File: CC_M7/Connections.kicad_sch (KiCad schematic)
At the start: 11 parts, among them J11 USB_B_Micro, J12 Conn_01x05_Pin, J16 Conn_01x06_Pin, J17 Conn_01x04_Pin, J3 Conn_01x03_Pin, J4 Conn_01x03_Pin, J5 Conn_01x03_Pin, J6 Conn_01x03_Pin, J7 Conn_01x03_Pin, J8 Conn_01x03_Pin

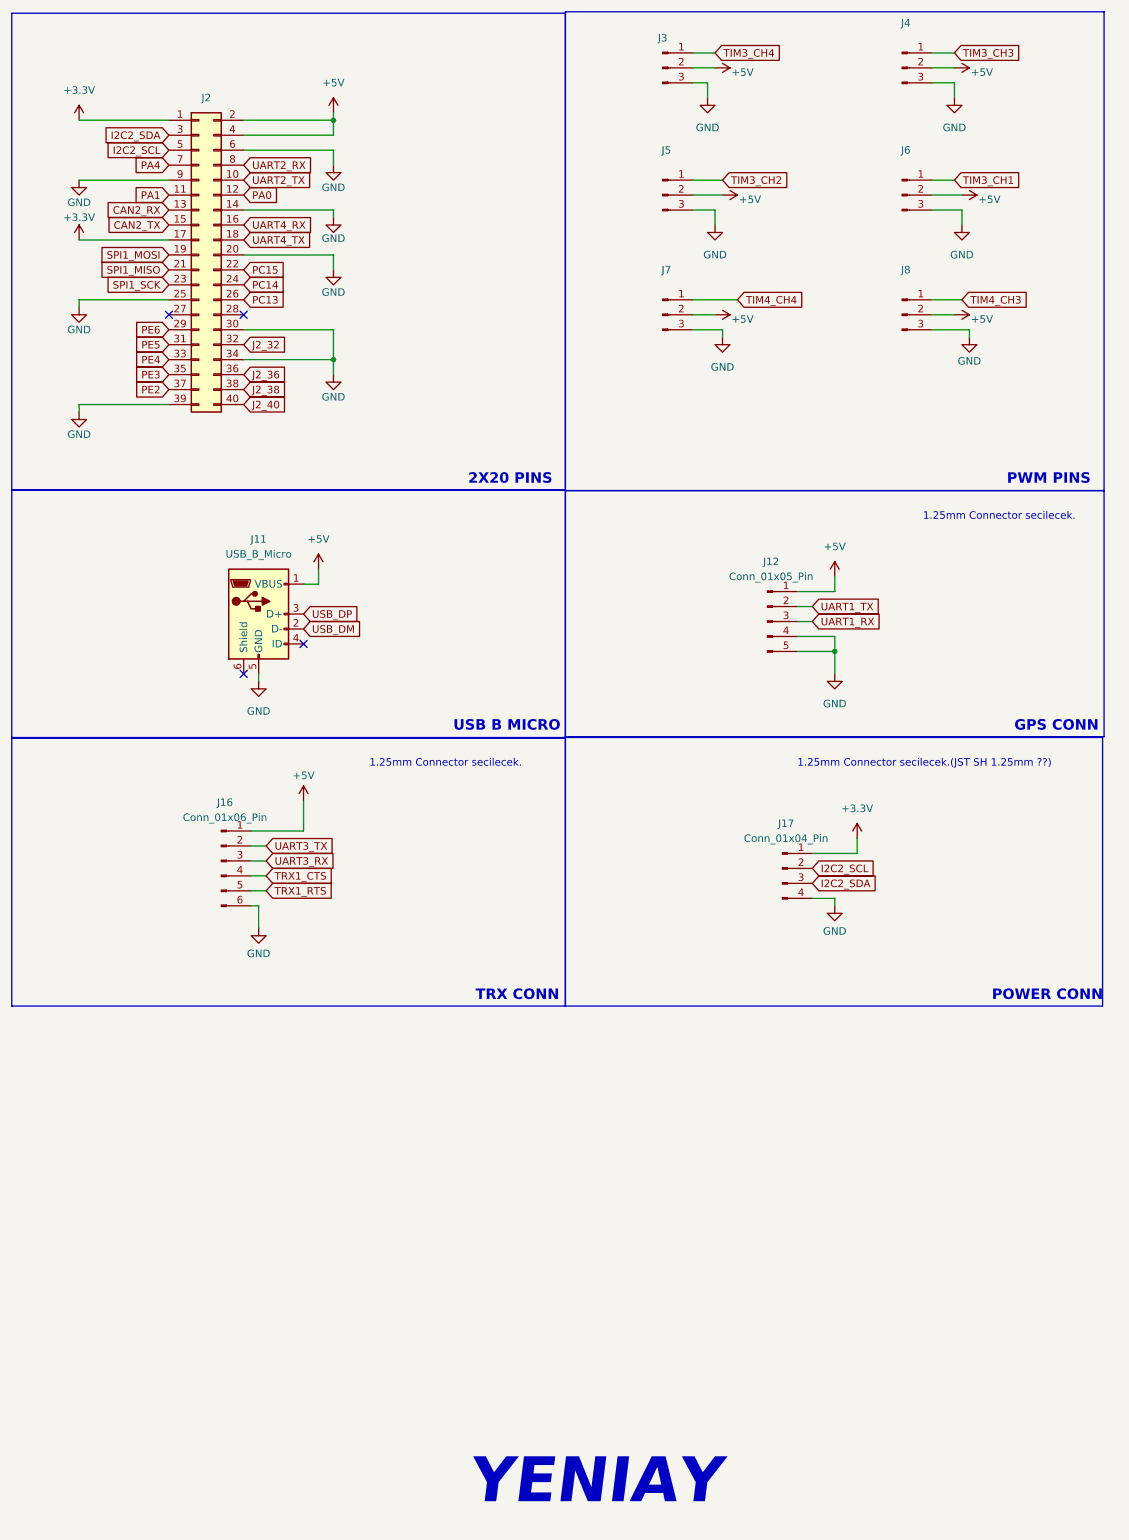
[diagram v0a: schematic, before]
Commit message: Changes updated @ CCM7.docx
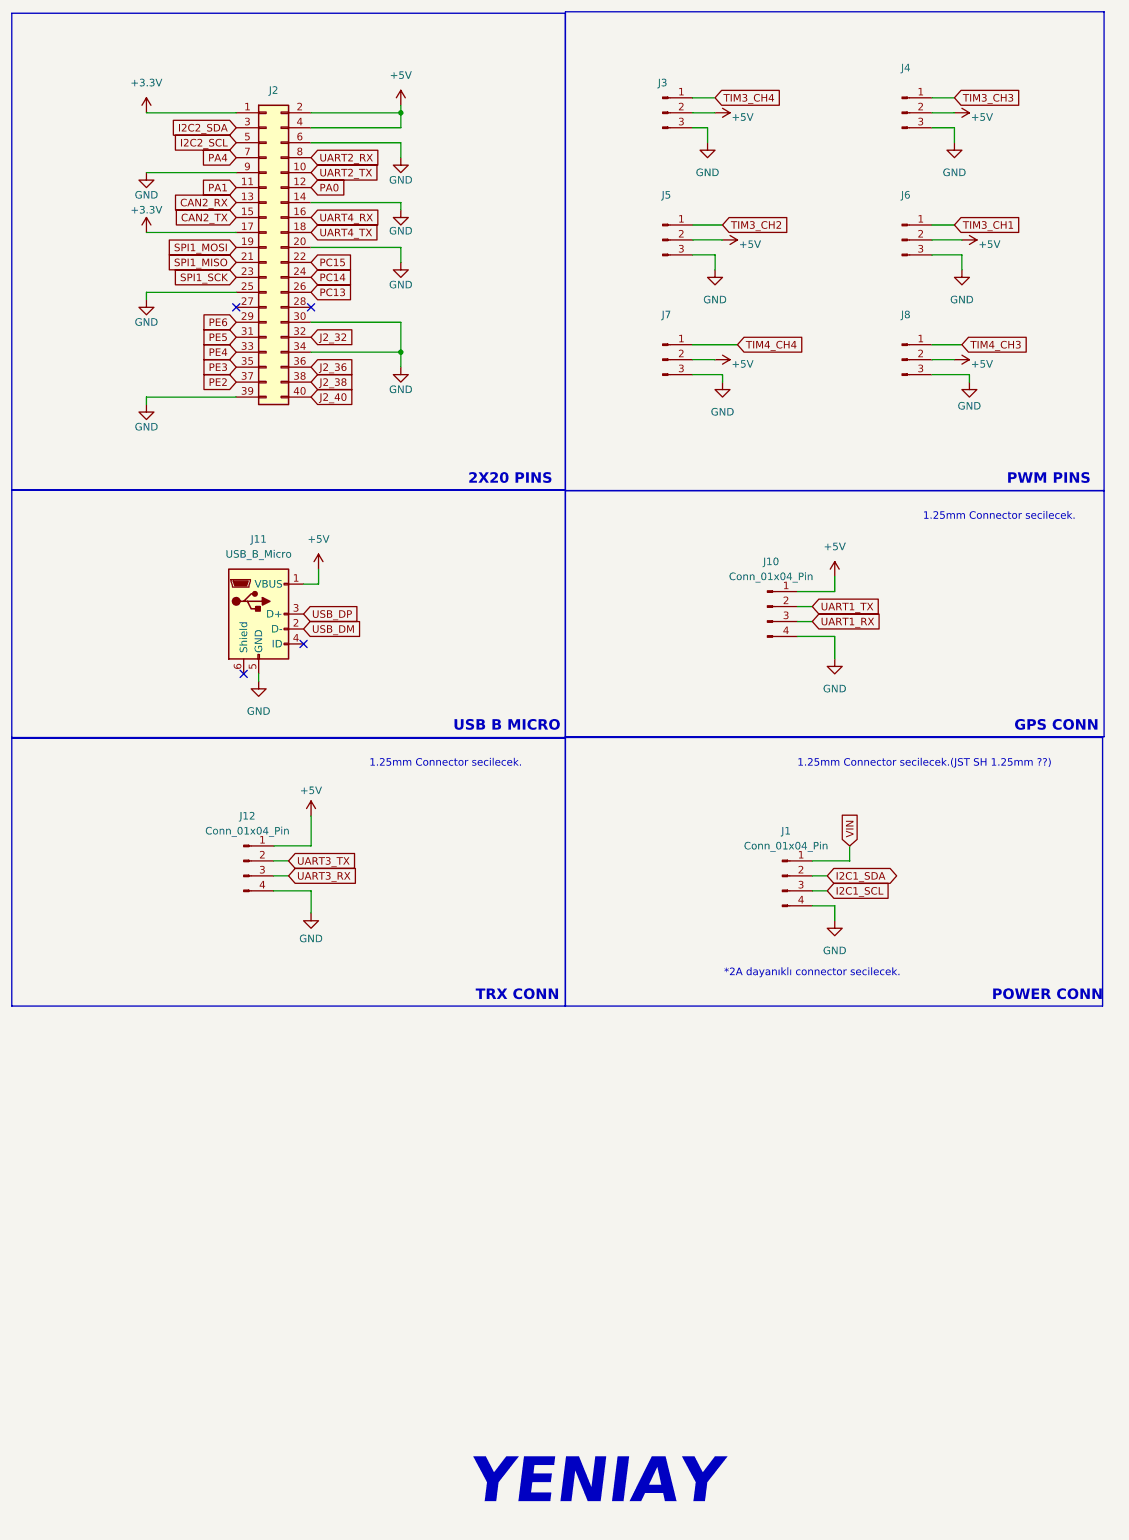
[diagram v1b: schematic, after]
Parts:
- removed J12: Conn_01x05_Pin, symbol Connector:Conn_01x05_Pin
- removed J16: Conn_01x06_Pin, symbol Connector:Conn_01x06_Pin
- removed J17: Conn_01x04_Pin, symbol Connector:Conn_01x04_Pin
- added J1, J10, J12: Conn_01x04_Pin, symbol Connector:Conn_01x04_Pin
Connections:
- net +5V: now also J10.1 (Pin_1), J12.1 (Pin_1)
- net GND: now also J1.4 (Pin_4), J10.4 (Pin_4), J12.4 (Pin_4)
- net UART1_RX: now also J10.3 (Pin_3)
- net UART1_TX: now also J10.2 (Pin_2)
- net UART3_RX: now also J12.3 (Pin_3)
- net UART3_TX: now also J12.2 (Pin_2)
- new net I2C1_SCL: J1.3 (Pin_3)
- new net I2C1_SDA: J1.2 (Pin_2)
- new net VIN: J1.1 (Pin_1)
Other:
- note added: "*2A dayanıklı connector secilecek."
- moved on the sheet: J2, J3, J4, J5, J6, J7, J8
